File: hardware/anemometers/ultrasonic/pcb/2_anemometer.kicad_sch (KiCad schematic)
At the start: 77 parts, among them Q2 SI2301CDS-T1-GE3, U4 MAX3222EIPWR, U5 SN74LV4052APW, U6 MAX3222EIPWR, U7 LMV358B-VR

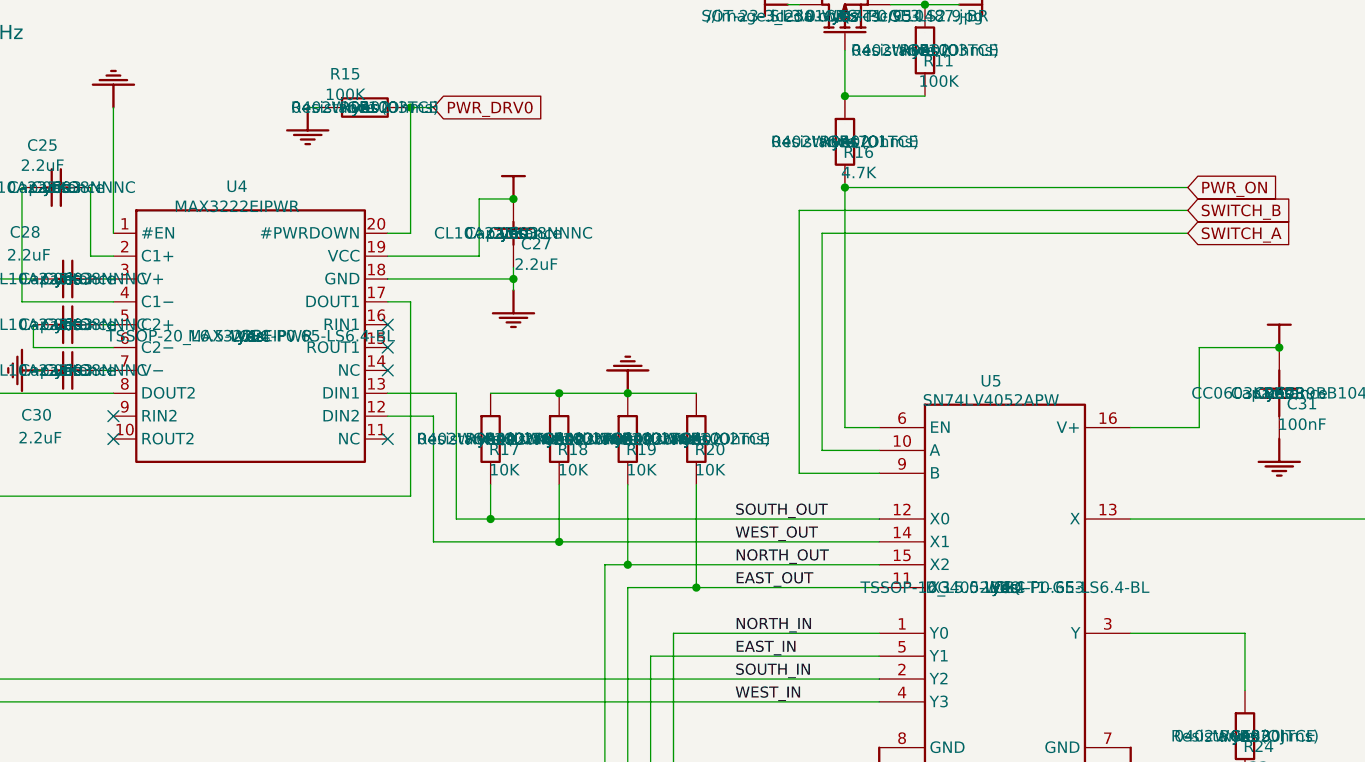
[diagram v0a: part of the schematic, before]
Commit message: Fix mux
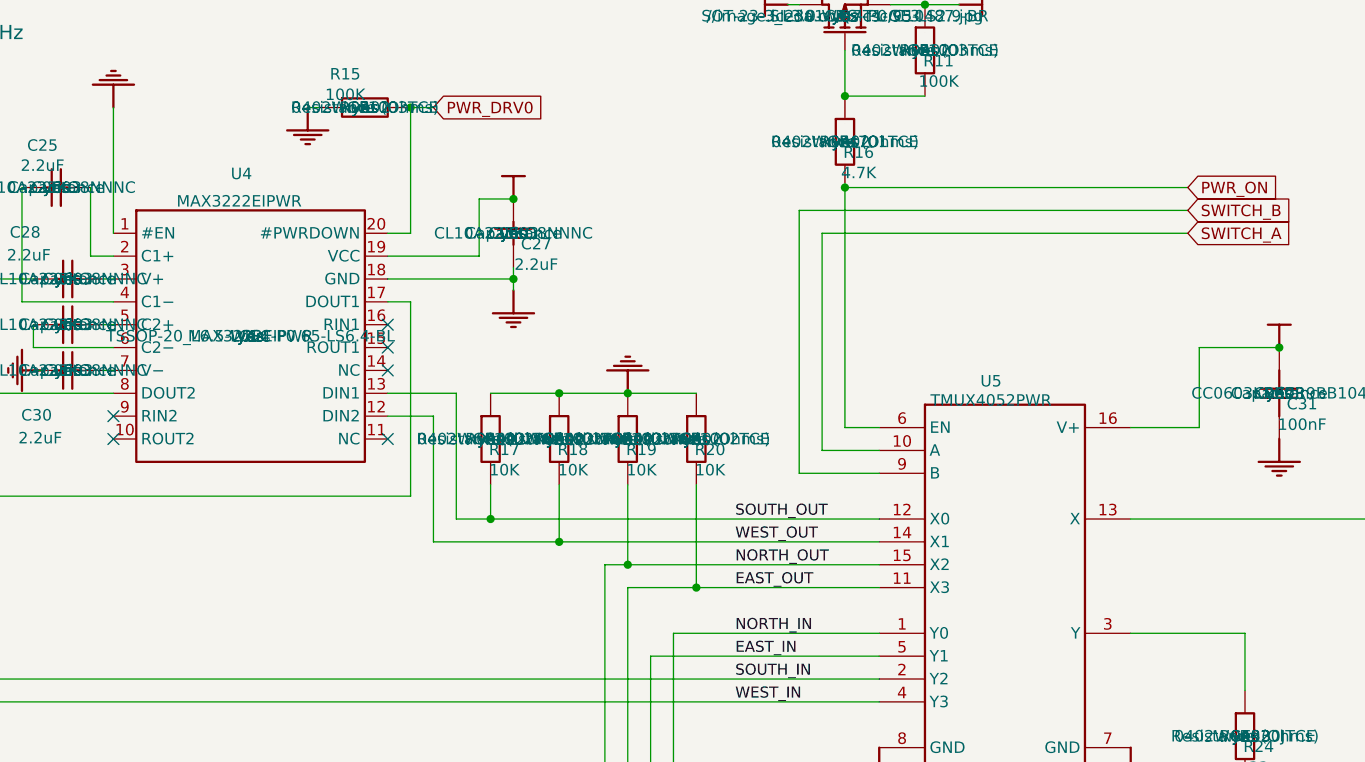
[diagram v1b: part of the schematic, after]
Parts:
- U5: value SN74LV4052APW -> TMUX4052PWR; Manufacturer VISHAY -> TI; Manufacturer Part SN74LV4052APW -> TMUX4052PWR; Supplier Part C145484 -> C7362466
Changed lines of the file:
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@@
 		(dnp no)
 		(property "Reference" "U4"
-			(at 187.706 79.9084 0)
+			(at 188.214 78.486 0)
 			(effects
 				(font
@@
 		)
 		(property "Value" "MAX3222EIPWR"
-			(at 187.706 82.1436 0)
+			(at 187.96 81.534 0)
 			(effects
 				(font
@@
 			)
 		)
-		(property "Value" "SN74LV4052APW"
+		(property "Value" "TMUX4052PWR"
 			(at 271.5006 103.6574 0)
 			(effects
@@
 			)
 		)
-		(property "Manufacturer Part" "SN74LV4052APW"
+		(property "Manufacturer Part" "TMUX4052PWR"
 			(at 273.05 124.46 0)
 			(effects
@@
 			)
 		)
-		(property "Manufacturer" "VISHAY"
+		(property "Manufacturer" "TI"
 			(at 273.05 124.46 0)
 			(effects
@@
 			)
 		)
-		(property "Supplier Part" "C145484"
+		(property "Supplier Part" "C7362466"
 			(at 273.05 124.46 0)
 			(effects
@@
 					(size 1.27 1.27)
 				)
+				(hide yes)
 			)
 		)
@@
 					(size 1.27 1.27)
 				)
+				(hide yes)
 			)
 		)
@@
 					(size 1.27 1.27)
 				)
+				(hide yes)
 			)
 		)
@@
 					(size 1.27 1.27)
 				)
+				(hide yes)
 			)
 		)
@@
 					(size 1.27 1.27)
 				)
+				(hide yes)
 			)
 		)
@@
 					(size 1.27 1.27)
 				)
+				(hide yes)
 			)
 		)

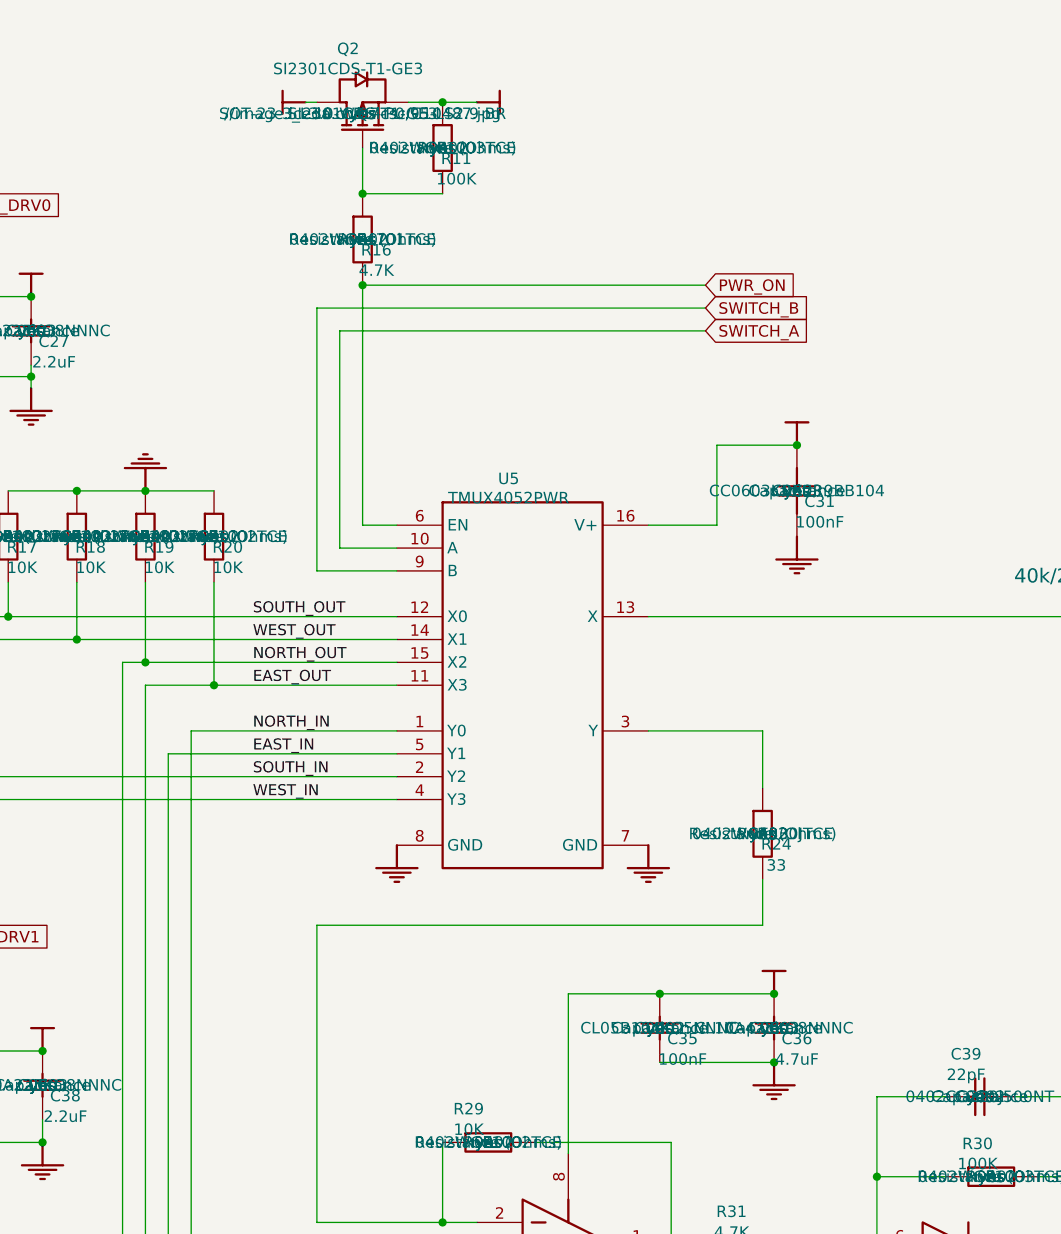
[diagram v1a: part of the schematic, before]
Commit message: Fixes!
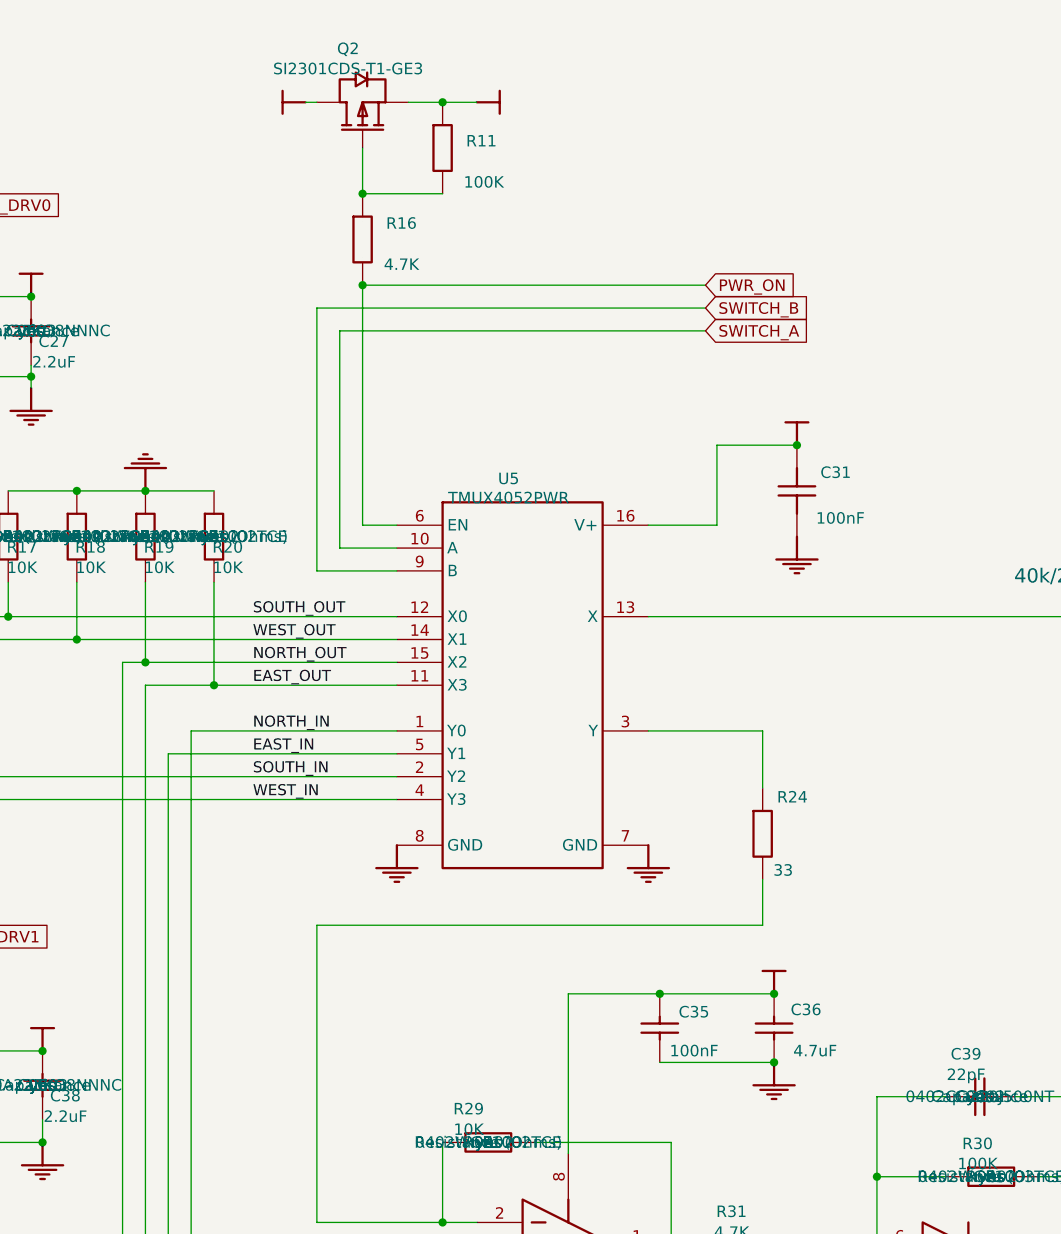
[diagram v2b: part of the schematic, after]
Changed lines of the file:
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@@
 		(dnp no)
 		(property "Reference" "R24"
-			(at 301.244 142.1384 90)
+			(at 303.022 136.906 90)
 			(effects
 				(font
@@
 		)
 		(property "Value" "33"
-			(at 301.244 144.4752 90)
+			(at 302.006 145.034 90)
 			(effects
 				(font
@@
 					(size 1.27 1.27)
 				)
+				(hide yes)
 			)
 		)
@@
 					(size 1.27 1.27)
 				)
+				(hide yes)
 			)
 		)
@@
 					(size 1.27 1.27)
 				)
+				(hide yes)
 			)
 		)
@@
 					(size 1.27 1.27)
 				)
+				(hide yes)
 			)
 		)
@@
 					(size 1.27 1.27)
 				)
+				(hide yes)
 			)
 		)
@@
 					(size 1.27 1.27)
 				)
+				(hide yes)
 			)
 		)
@@
 		(dnp no)
 		(property "Reference" "R11"
-			(at 265.684 65.9638 90)
+			(at 268.478 64.008 90)
 			(effects
 				(font
@@
 		)
 		(property "Value" "100K"
-			(at 265.684 68.2244 90)
+			(at 268.732 68.58 90)
 			(effects
 				(font
@@
 					(size 1.27 1.27)
 				)
+				(hide yes)
 			)
 		)
@@
 					(size 1.27 1.27)
 				)
+				(hide yes)
 			)
 		)
@@
 					(size 1.27 1.27)
 				)
+				(hide yes)
 			)
 		)
@@
 					(size 1.27 1.27)
 				)
+				(hide yes)
 			)
 		)
@@
 					(size 1.27 1.27)
 				)
+				(hide yes)
 			)
 		)
@@
 					(size 1.27 1.27)
 				)
+				(hide yes)
 			)
 		)
@@
 		(dnp no)
 		(property "Reference" "C36"
-			(at 303.53 163.7538 90)
+			(at 304.546 160.528 90)
 			(effects
 				(font
@@
 		)
 		(property "Value" "4.7uF"
-			(at 303.53 166.0398 90)
+			(at 305.562 165.1 90)
 			(effects
 				(font
@@
 					(size 1.27 1.27)
 				)
+				(hide yes)
 			)
 		)
@@
 					(size 1.27 1.27)
 				)
+				(hide yes)
 			)
 		)
@@
 					(size 1.27 1.27)
 				)
+				(hide yes)
 			)
 		)
@@
 					(size 1.27 1.27)
 				)
+				(hide yes)
 			)
 		)
@@
 					(size 1.27 1.27)
 				)
+				(hide yes)
 			)
 		)
@@
 					(size 1.27 1.27)
 				)
+				(hide yes)
 			)
 		)
@@
 		(dnp no)
 		(property "Reference" "C31"
-			(at 306.07 104.0638 90)
+			(at 307.848 100.838 90)
 			(effects
 				(font
@@
 		)
 		(property "Value" "100nF"
-			(at 306.07 106.3498 90)
+			(at 308.356 105.918 90)
 			(effects
 				(font
@@
 					(size 1.27 1.27)
 				)
+				(hide yes)
 			)
 		)
@@
 					(size 1.27 1.27)
 				)
+				(hide yes)
 			)
 		)
@@
 					(size 1.27 1.27)
 				)
+				(hide yes)
 			)
 		)
@@
 					(size 1.27 1.27)
 				)
+				(hide yes)
 			)
 		)
@@
 					(size 1.27 1.27)
 				)
+				(hide yes)
 			)
 		)
@@
 					(size 1.27 1.27)
 				)
+				(hide yes)
 			)
 		)
@@
 		(dnp no)
 		(property "Reference" "C35"
-			(at 290.83 163.7538 90)
+			(at 292.1 160.782 90)
 			(effects
 				(font
@@
 		)
 		(property "Value" "100nF"
-			(at 290.83 166.0398 90)
+			(at 292.1 165.1 90)
 			(effects
 				(font
@@
 					(size 1.27 1.27)
 				)
+				(hide yes)
 			)
 		)
@@
 					(size 1.27 1.27)
 				)
+				(hide yes)
 			)
 		)
@@
 					(size 1.27 1.27)
 				)
+				(hide yes)
 			)
 		)
@@
 					(size 1.27 1.27)
 				)
+				(hide yes)
 			)
 		)
@@
 					(size 1.27 1.27)
 				)
+				(hide yes)
 			)
 		)
@@
 					(size 1.27 1.27)
 				)
+				(hide yes)
 			)
 		)
@@
 					(size 1.27 1.27)
 				)
+				(hide yes)
 			)
 		)
@@
 					(size 1.27 1.27)
 				)
+				(hide yes)
 			)
 		)
@@
 					(size 1.27 1.27)
 				)
+				(hide yes)
 			)
 		)
@@
 					(size 1.27 1.27)
 				)
+				(hide yes)
 			)
 		)
@@
 					(size 1.27 1.27)
 				)
+				(hide yes)
 			)
 		)
@@
 					(size 1.27 1.27)
 				)
+				(hide yes)
 			)
 		)
@@
 		(dnp no)
 		(property "Reference" "R16"
-			(at 256.794 76.1238 90)
+			(at 259.588 73.152 90)
 			(effects
 				(font
@@
 		)
 		(property "Value" "4.7K"
-			(at 256.794 78.3844 90)
+			(at 259.588 77.724 90)
 			(effects
 				(font
@@
 					(size 1.27 1.27)
 				)
+				(hide yes)
 			)
 		)
@@
 					(size 1.27 1.27)
 				)
+				(hide yes)
 			)
 		)
@@
 					(size 1.27 1.27)
 				)
+				(hide yes)
 			)
 		)
@@
 					(size 1.27 1.27)
 				)
+				(hide yes)
 			)
 		)
@@
 					(size 1.27 1.27)
 				)
+				(hide yes)
 			)
 		)
@@
 					(size 1.27 1.27)
 				)
+				(hide yes)
 			)
 		)
